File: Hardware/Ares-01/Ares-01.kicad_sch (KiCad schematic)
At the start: 26 parts, among them J1 BTS7960, J12 XT30, J13 TCRT5000_1, J14 TCRT5000_2, J15 TCRT5000_3, J2 BTS7960, J3 Sharp, J4 Sharp, J5 Sharp, J6 Sharp, J7 Sharp, J8 Qtr8a, J9 Ssd1306 Arduino Pic, SW1 Switch, SW2 SW_Push, SW3 SW_Push, U1 L7805, U2 AMS1117, U3 CD74HC4067M

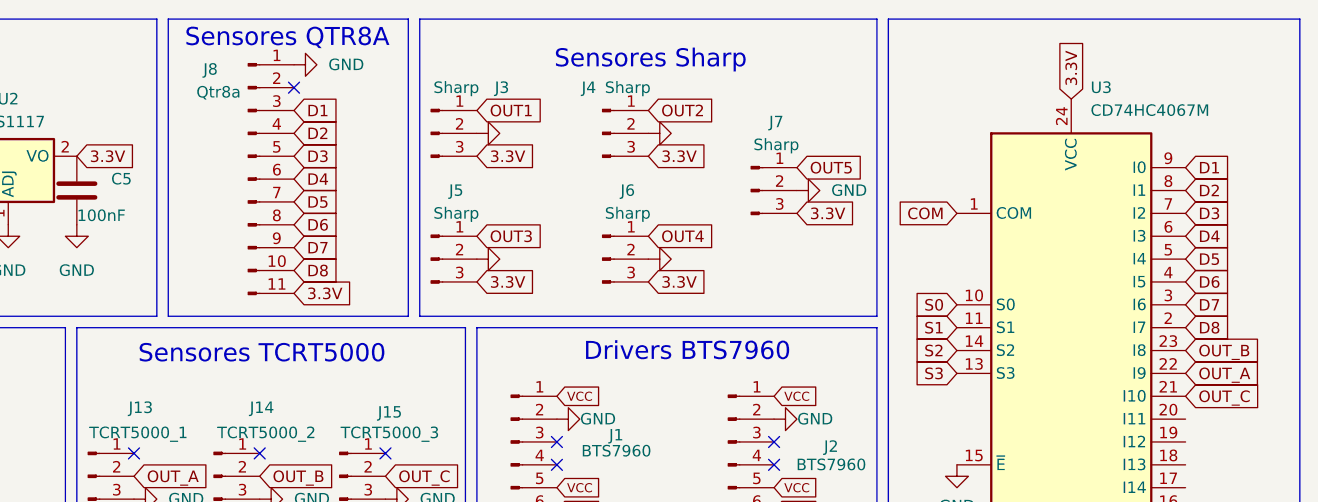
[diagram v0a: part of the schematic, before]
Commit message: Se actualizo PCB
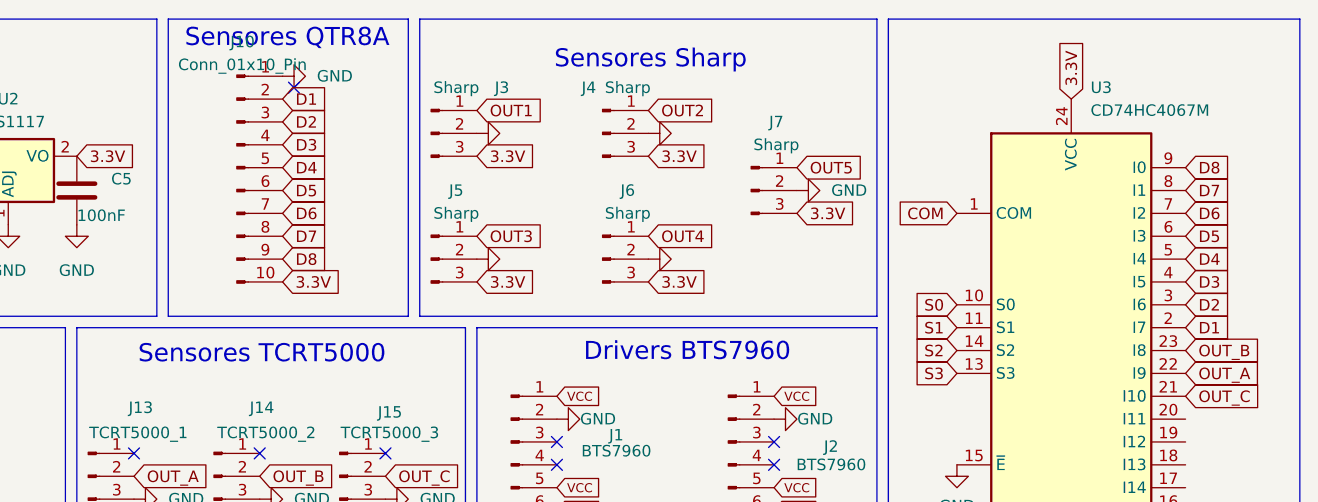
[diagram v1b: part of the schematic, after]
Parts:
- removed J8: Qtr8a, Connector_JST:JST_XH_B10B-XH-A_1x10_P2.50mm_Vertical, symbol Connector:Conn_01x11_Pin
- added J10: Conn_01x10_Pin, Connector_JST:JST_XH_B10B-XH-A_1x10_P2.50mm_Vertical, symbol Connector:Conn_01x10_Pin
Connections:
- net 3.3V: now also J10.10 (Pin_10)
- net D1: now also U3.2 (I7), J10.2 (Pin_2); no longer U3.9 (I0)
- net D2: now also U3.3 (I6), J10.3 (Pin_3); no longer U3.8 (I1)
- net D3: now also U3.4 (I5), J10.4 (Pin_4); no longer U3.7 (I2)
- net D4: now also U3.5 (I4), J10.5 (Pin_5); no longer U3.6 (I3)
- net D5: now also U3.6 (I3), J10.6 (Pin_6); no longer U3.5 (I4)
- net D6: now also U3.7 (I2), J10.7 (Pin_7); no longer U3.4 (I5)
- net D7: now also U3.8 (I1), J10.8 (Pin_8); no longer U3.3 (I6)
- net D8: now also U3.9 (I0), J10.9 (Pin_9); no longer U3.2 (I7)
- net GND: now also J10.1 (Pin_1)
